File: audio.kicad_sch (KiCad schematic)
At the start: 69 parts, among them U10 OPA1642, U17 DG413xUE, U4 OPA1692xD, U5 OPA1692xD, U7 OPA1692xD, U8 OPA1692xD, U9 OPA1692xD

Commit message: modified:   MCU.kicad_sch 	modified:   PSU.kicad_sch 	modified:   ProjectY.kicad_pro 	modified:   ProjectY.kicad_sch 	modified:   ad.kicad_sch 	modified:   audio.kicad_sch
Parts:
- removed R25, R26: 4.7k, symbol Device:R
- removed U10: OPA1642, Package_SO:SOIC-8_3.9x4.9mm_P1.27mm, symbol Amplifier_Operational:OPA1692xD
- removed U17: DG413xUE, Package_SO:TSSOP-16_4.4x5mm_P0.65mm, symbol Analog_Switch:DG413xUE
- removed U9: OPA1692xD, Package_SO:SOIC-8_3.9x4.9mm_P1.27mm, symbol Amplifier_Operational:OPA1692xD
- added C1: 10u, symbol Device:C_Polarized
- added C13, C23: 1uF, PCM_JLCPCB:C_0402, symbol PCM_JLCPCB-Capacitors:0402,1uF
- added C21, C22: 10uF, PCM_JLCPCB:C_0402, symbol PCM_JLCPCB-Capacitors:0402,10uF
- added U6: TAC5242, Package_DFN_QFN:VQFN-24-1EP_4x4mm_P0.5mm_EP2.5x2.5mm_ThermalVias, symbol User:TAC5242
- added U9: OPA2156xD, Package_SO:SOIC-8_3.9x4.9mm_P1.27mm, symbol Amplifier_Operational:OPA2156xD
- R19, R20: value 4.7k -> 10k
- R23, R24: value 4.7k -> 2Meg
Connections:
- net VREF is gone; now on net +3.5VA: U8.3 (+), U8.5 (+)
- net ADC_L+: now also U6.15 (IN1P)
- net ADC_L-: now also U6.16 (IN1M)
- net ADC_R+: now also U6.17 (IN2P)
- net ADC_R-: now also U6.18 (IN2M)
- net DAC_L+: now also U6.20 (OUT1P)
- net DAC_L-: now also U6.19 (OUT1M)
- net DAC_R+: now also U6.21 (OUT2P)
- net DAC_R-: now also U6.22 (OUT2M)
- net GND: now also R20.2, R23.2, R24.2, C1.2, C13.2, C21.2, C22.2, C23.2, U6.10 (MD4), U6.12 (MD5), U6.13 (MD0), U6.25 (EPAD), U6.9 (MD3), U6.A1 (VSS), U6.A2 (VSS), U6.A3 (VSS), U6.A4 (VSS), U9.4 (V-); no longer R22.2, R28.2, R30.2, R32.2, R34.2, R8.2
- net Guitar_IN_L: now also R23.1
- net Guitar_IN_R: now also R24.1
- net at C34.2, R3.2, U7.1: now also R41.1; no longer R20.1
- net at C31.2, R14.2, R8.1: now also U9.3 (+)
- net at R15.1, R27.1: now also U9.1, U9.2 (-)
- net at C33.2, R21.2, R22.1: now also U9.5 (+)
- net at R17.1, R31.1: now also U9.6 (-), U9.7
- net at C39.2, R13.2, U7.7: now also R42.1; no longer R24.1
- net +3.5VA: now reaches R19.2
- net +3.5VA: now also R20.1, R22.2, R28.2, R30.2, R32.2, R34.2, R8.2, C1.1; no longer R41.1
- net +7VA: now reaches R19.1
- net +7VA: now also U9.8 (V+); no longer R20.2
- net ADC_DRV_OUT_L-: no longer names the net of R16.1, R29.1, U8.1
- net ADC_DRV_OUT_L-: no longer R23.2
- net ADC_DRV_OUT_R-: no longer names the net of R18.1, R33.1, U8.7
- new net: C13.1, U6.14 (MICBIAS)
- new net: C22.1, U6.1 (DREG)
- new net: C23.1, U6.24 (VREF)
- new net 3.3V: C21.1, U6.6 (IOVDD)
- new net 3.3VA: U6.23 (AVDD), U6.7 (MD1), U6.8 (MD2)
- new net GP0: U6.11 (GPO)
- new net I2S_CK: U6.2 (BCLK)
- new net I2S_SDI: U6.4 (DOUT)
- new net I2S_SDO: U6.5 (DIN)
- new net I2S_WS: U6.3 (FSYNC)
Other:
- moved on the sheet: C27, C28, C29, C30, C34, C35, C36, C37, C38, C39, R1, R10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

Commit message: modified:   MCU.kicad_sch 	modified:   PSU.kicad_sch 	modified:   ProjectY.kicad_pro 	modified:   ProjectY.kicad_sch 	modified:   audio.kicad_sch 	modified:   fp-info-cache 	new file:   spdif.kicad_sch 	modified:   usbfilter.kicad_sch
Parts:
- removed C1: 10u, symbol Device:C_Polarized
- removed C34, C38, C39: 330p, symbol Device:C
- removed C35, C36: 100u, symbol Device:C
- removed C37, C44, C45: 2.2n, symbol Device:C
- removed R10, R13: 4.7k, symbol Device:R
- removed R11, R12: 200, symbol Device:R
- removed R19, R20: 10k, symbol Device:R
- removed R45, R46: 100, symbol Device:R
- removed U4, U5, U7, U8: OPA1692xD, Package_SO:SOIC-8_3.9x4.9mm_P1.27mm, symbol Amplifier_Operational:OPA1692xD
- added C1, C11, C12, C15, C16, C17, C18, C19, C2, C20: 100nF, PCM_JLCPCB:C_0402, symbol PCM_JLCPCB-Capacitors:0402,100nF
- added C36, C37, C38, C39, C44, C45: 2.2nF, PCM_JLCPCB:C_0805, symbol PCM_JLCPCB-Capacitors:0805,2.2nF
- added D2, D3, D4, D5, D6, D7: BAV99,215, PCM_JLCPCB:SOT-23-3_L2.9-W1.6-P1.90-LS2.8-BR, symbol PCM_JLCPCB-Diode-Packages:Switching, BAV99,215
- added R43, R44: 600 0.1%, symbol Device:R
- added U10, U14: OPA1692xDGK, Package_SO:VSSOP-8_3x3mm_P0.65mm, symbol Amplifier_Operational:OPA1692xDGK
- added U7, U8: OPA2156xD, Package_SO:SOIC-8_3.9x4.9mm_P1.27mm, symbol Amplifier_Operational:OPA2156xD
- C29: value 2.2n -> 100u
- C30: value 330p -> 100u
- R1, R2: value 4.7k -> 1k 0.1%
- R15, R16, R17, R18: value 4.7k -> 2.2k
- R27, R28, R29, R30, R31, R32, R33, R34: value 2.2k -> 1k
- R3, R6, R7, R9: value 4.7k -> ?
- R4, R5: value 200 -> 1k 0.1%
- R41, R42: value 100 -> 600 0.1%
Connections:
- net +3.5VA: now also U8.3 (+), U8.5 (+); no longer R22.2, R28.2, R30.2, R32.2, R34.2, R8.2
- net DAC_R+: now also C30.2
- net DAC_R-: now also C29.1
- net GND: now also R22.2, R28.2, R30.2, R32.2, R34.2, R42.1, R7.1, R8.2, C1.2, C11.2, C12.1, C15.2, C16.1, C17.2, C18.1, C19.2, C2.1, C20.1, R44.1; no longer C30.2, U9.4 (V-)
- net Guitar_IN_L: now also D2.3
- net Guitar_IN_R: now also D3.3
- net Line_Output_L+: now also D4.3
- net Line_Output_L-: now also R42.2, D5.3
- net Line_Output_R+: now also D6.3, R43.2; no longer R42.2
- net Line_Output_R-: now also D7.3, R44.2
- net at R1.2, R3.1: now also C38.2, C39.2, U7.2 (-); no longer C29.1, R4.1
- net at R3.2, R41.1: now also U7.1
- net at R27.2, R28.1: now also U10.5 (+)
- net at R7.2: now also R5.2, C44.1, C45.1, U7.5 (+)
- net at R31.2, R32.1: now also U14.5 (+)
- net at R2.2, R6.2: now also C38.1, C39.1, U7.3 (+); no longer C29.2, R5.1
- net at C46.1, R37.2: now also C37.2
- net at C47.2, R38.2: now also C37.1
- net at R4.2: now also R9.1, C44.2, C45.2, U7.6 (-)
- net at R18.1, R33.1: now also U8.7
- net at R33.2, R34.1: now also U14.3 (+)
- net at R9.2: now also R43.1, U7.7
- net at R16.1, R29.1: now also U8.1
- net at R15.2, R16.2: now also U8.2 (-)
- net at R37.1: now also U14.1, U14.2 (-)
- net at R29.2, R30.1: now also U10.3 (+)
- net at R38.1: now also U14.6 (-), U14.7
- net at R17.2, R18.2: now also U8.6 (-)
- net at C30.1: now also R5.1; no longer R5.2
- net at C40.1, R35.2: now also C36.2
- net at C43.2, R36.2: now also C36.1
- net at R36.1: now also U10.6 (-), U10.7
- net at R35.1: now also U10.1, U10.2 (-)
- net +7VA renamed +5V
- net +5V: now also C1.1, C11.1, C15.1, C17.1, C19.1, D2.2, D3.2, D4.2, D5.2, D6.2, D7.2, U10.8 (V+), U14.8 (V+), U7.8 (V+), U8.8 (V+)
- new net: C29.2, R4.1
- new net -5V: C12.2, C16.2, C18.2, C2.2, C20.2, D2.1, D3.1, D4.1, D5.1, D6.1, D7.1, U10.4 (V-), U14.4 (V-), U7.4 (V-), U8.4 (V-), U9.4 (V-)
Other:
- moved on the sheet: C13, C21, C22, C23, C27, C28, C31, C32, C33, C40, C43, C46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

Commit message: asd
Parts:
- removed C31, C33: 100p, symbol Device:C
- removed C32, C8: 1u, symbol Device:C
- removed D2, D3, D4, D5, D6, D7: BAV99,215, PCM_JLCPCB:SOT-23-3_L2.9-W1.6-P1.90-LS2.8-BR, symbol PCM_JLCPCB-Diode-Packages:Switching, BAV99,215
- removed R1, R2, R4, R5: 1k 0.1%, symbol Device:R
- removed R14, R21, R35, R36, R37, R38: 100, symbol Device:R
- removed R15, R16, R17, R18: 2.2k, symbol Device:R
- removed R22, R23, R24, R8: 2Meg, symbol Device:R
- removed R27, R28, R29, R30, R31, R32, R33, R34: 1k, symbol Device:R
- removed U7: OPA2156xD, Package_SO:SOIC-8_3.9x4.9mm_P1.27mm, symbol Amplifier_Operational:OPA2156xD
- added C31, C32, C70, C71, C72, C8, C81, C82, C83, C84: 100nF, PCM_JLCPCB:C_0402, symbol PCM_JLCPCB-Capacitors:0402,100nF
- added C34, C35, C85, C86, C87, C94: 100pF, PCM_JLCPCB:C_0402, symbol PCM_JLCPCB-Capacitors:0402,100pF
- added D11, D12, D13, D14, D15, D16, D17, D18, D19, D8: BAV99, Package_TO_SOT_SMD:SOT-23, symbol Diode:BAV99
- added K1, K2, K3, K4: G6K-2, symbol Relay:G6K-2
- added Q6, Q7, Q8, Q9: BC847, Package_TO_SOT_SMD:SOT-23, symbol Transistor_BJT:BC847
- added R100, R103, R68, R71: 10kΩ, PCM_JLCPCB:R_0402, symbol PCM_JLCPCB-Resistors:0402,10kΩ
- added R101, R102, R20, R21, R22, R23, R26, R27, R28, R29, R31, R32, R33, R34, R37, R38, R62, R63, R64, R65, R66, R67, R72, R73, R76, R77: 1kΩ, PCM_JLCPCB:R_0805, symbol PCM_JLCPCB-Resistors:0805,1kΩ
- added R13, R14, R16, R24, R25, R69, R70, R80, R81, R98: 100Ω, PCM_JLCPCB:R_0805, symbol PCM_JLCPCB-Resistors:0805,100Ω
- added R17, R18: 2.2kΩ, PCM_JLCPCB:R_0805, symbol PCM_JLCPCB-Resistors:0805,2.2kΩ
- added R75, R79, R82, R83: 510Ω, PCM_JLCPCB:R_0805, symbol PCM_JLCPCB-Resistors:0805,510Ω
- added R8, R99: 1MΩ, PCM_JLCPCB:R_0805, symbol PCM_JLCPCB-Resistors:0805,1MΩ
- added R88, R89, R90, R91: 10kΩ, PCM_JLCPCB:R_0805, symbol PCM_JLCPCB-Resistors:0805,10kΩ
- added U13, U16, U23, U5: OPA2156xD, Package_SO:SOIC-8_3.9x4.9mm_P1.27mm, symbol Amplifier_Operational:OPA2156xD
- added U24: OPA1692xDGK, Package_SO:VSSOP-8_3x3mm_P0.65mm, symbol Amplifier_Operational:OPA1692xDGK
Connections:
- net +3.5VA is gone; now on net GND: U8.3 (+), U8.5 (+)
- net DAC_R+: now also C29.1; no longer C30.2
- net DAC_R-: now also C30.2; no longer C29.1
- net GND: now also C31.2, C32.1, C34.2, C35.2, C70.2, C71.1, C72.2, C8.2, C81.1, C82.2, C83.1, C84.1, C85.2, C86.2, C87.2, C94.2, Q6.2 (E), Q7.2 (E), Q8.2 (E), Q9.2 (E), R20.2, R23.2, R32.2, R34.2, R79.1, R8.2, R83.2, R88.2, R89.1, R90.2, R91.1, R99.2, U5.3 (+), U5.5 (+)
- net Line_Output_L+: now also D12.3 (K)
- net Line_Output_L-: now also D13.3 (K)
- net Line_Output_R+: now also D14.3 (K)
- net Line_Output_R-: now also D15.3 (K)
- net at C38.2, C39.2, R3.1: now also R26.2, U24.2 (-)
- net at R3.2: now also R62.2, U24.1; no longer R41.1
- net at C38.1, C39.1, R6.2: now also R27.2, U24.3 (+)
- net at U9.3 (+): now also C34.1, R13.2, R8.1
- net Unbal_Left: now reaches U9.1, U9.2 (-)
- net Unbal_Left: now also K2.5
- net at U10.5 (+): now also R20.1, R21.2
- net at U9.5 (+): now also C94.1, R98.2, R99.1
- net at C44.2, C45.2, R9.1: now also R28.2, U24.6 (-)
- net at R9.2: now also R64.2, U24.7; no longer R43.1
- net Unbal_Right: now reaches U9.6 (-), U9.7
- net Unbal_Right: now also K2.4
- net at U14.5 (+): now also R33.2, R34.1
- net at C30.1: now also R29.1
- net at C27.2: now also R26.1
- net Processing_Inverted_Right: now reaches U8.7
- net Processing_Inverted_Right: now also R18.2, R31.1, R66.1
- net at U14.3 (+): now also R31.2, R32.1
- net at C44.1, C45.1, R7.2: now also R29.2, U24.5 (+)
- net Processing_Inverted_Left: now reaches U8.1
- net Processing_Inverted_Left: now also R101.1, R102.1, R22.1, R67.1, R77.2
- net at U8.2 (-): now also R76.1, R77.1
- net at U14.6 (-), U14.7: now also R70.1
- net at U10.3 (+): now also R22.2, R23.1
- net at U14.1, U14.2 (-): now also R69.1
- net at C37.2, C46.1: now also R69.2
- net at U10.6 (-), U10.7: now also R25.1
- net at C28.1: now also R27.1
- net at U8.6 (-): now also R17.2, R18.1
- net at C36.1, C43.2: now also R25.2
- net at C36.2, C40.1: now also R24.2
- net at C29.2: now also R28.1
- net at U10.1, U10.2 (-): now also R24.1
- net at C37.1, C47.2: now also R70.2
- net +5V renamed +4.5V
- net +4.5V: now also C31.1, C70.1, C72.1, C8.1, C82.1, D11.2 (A), D12.2 (A), D13.2 (A), D14.2 (A), D15.2 (A), D16.2 (A), D17.2 (A), D18.2 (A), D19.2 (A), D8.2 (A), U13.8 (V+), U16.8 (V+), U23.8 (V+), U24.8 (V+), U5.8 (V+)
- net -5V renamed -4.5V
- net -4.5V: now also C32.2, C71.2, C81.2, C83.2, C84.2, D11.1 (K), D12.1 (K), D13.1 (K), D14.1 (K), D15.1 (K), D16.1 (K), D17.1 (K), D18.1 (K), D19.1 (K), D8.1 (K), U13.4 (V-), U16.4 (V-), U23.4 (V-), U24.4 (V-), U5.4 (V-)
- net 3.3V renamed +3.3V
- net +3.3V: now also K1.1, K2.1, K3.1, K4.1
- net 3.3VA renamed +3.3VA
- new net: Q7.1 (B), R71.2
- new net: K2.8, Q7.3 (C)
- new net: C86.1, R80.2, R90.1, U23.3 (+)
- new net: R37.2, R75.1, U16.2 (-)
- new net: R38.2, R79.2, U16.3 (+)
- new net: C35.1, R14.2, R88.1, U13.3 (+)
- new net: C85.1, R16.2, R89.2, U13.5 (+)
- new net: R37.1, U13.1, U13.2 (-)
- new net: Q9.1 (B), R103.2
- new net: K4.8, Q9.3 (C)
- new net: C87.1, R81.2, R91.2, U23.5 (+)
- new net: R73.1, U23.6 (-), U23.7
- new net: K1.6, R66.2
- new net: Q8.1 (B), R68.2
- new net: K1.8, Q8.3 (C)
- new net: R43.1, R65.1, U5.1
- new net: R64.1, R65.2, U5.2 (-)
- new net: R72.1, U23.1, U23.2 (-)
- new net: Q6.1 (B), R100.2
- new net: R38.1, U13.6 (-), U13.7
- new net: R41.1, R63.1, U5.7
- new net: K4.3, R101.2
- new net: K4.6, R102.2
- new net: K1.3, R67.2
- new net: R73.2, R83.1, U16.5 (+)
- new net: K3.8, Q6.3 (C)
- new net: R72.2, R82.2, U16.6 (-)
- new net Balun_In_Left+: D16.3 (K), K3.5, R16.1
- new net Balun_In_Left-: D8.3 (K), K3.4, R14.1
- new net Balun_Left: K2.7, R75.2, U16.1
- new net Balun_Right: K2.2, R82.1, U16.7
- new net Buffer_In_Left: D11.3 (K), K3.7, R13.1
- new net Buffer_In_Right: D19.3 (K), K3.2, R98.1
- new net Dry_Through: R68.1
- new net Hi-Z: R71.1
- new net IN_L+: K3.6
- new net IN_L-: K3.3
- new net IN_R+: D18.3 (K), R81.1
- new net IN_R-: D17.3 (K), R80.1
- new net Mono_Dry_Through: R103.1
- new net Processing_In_Left: K2.6, R21.1, R76.2
- new net Processing_In_Right: K2.3, R17.1, R33.1
- new net Summing_In_L: K1.4, K4.4, R62.1, R63.2, U5.6 (-)
- new net Summing_In_R: K1.5, K4.5
- new net ~{Hi-Z2}: R100.1
- no-connect marks 0 -> 4
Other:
- moved on the sheet: C1, C11, C12, C13, C15, C16, C17, C18, C19, C2, C20, C21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

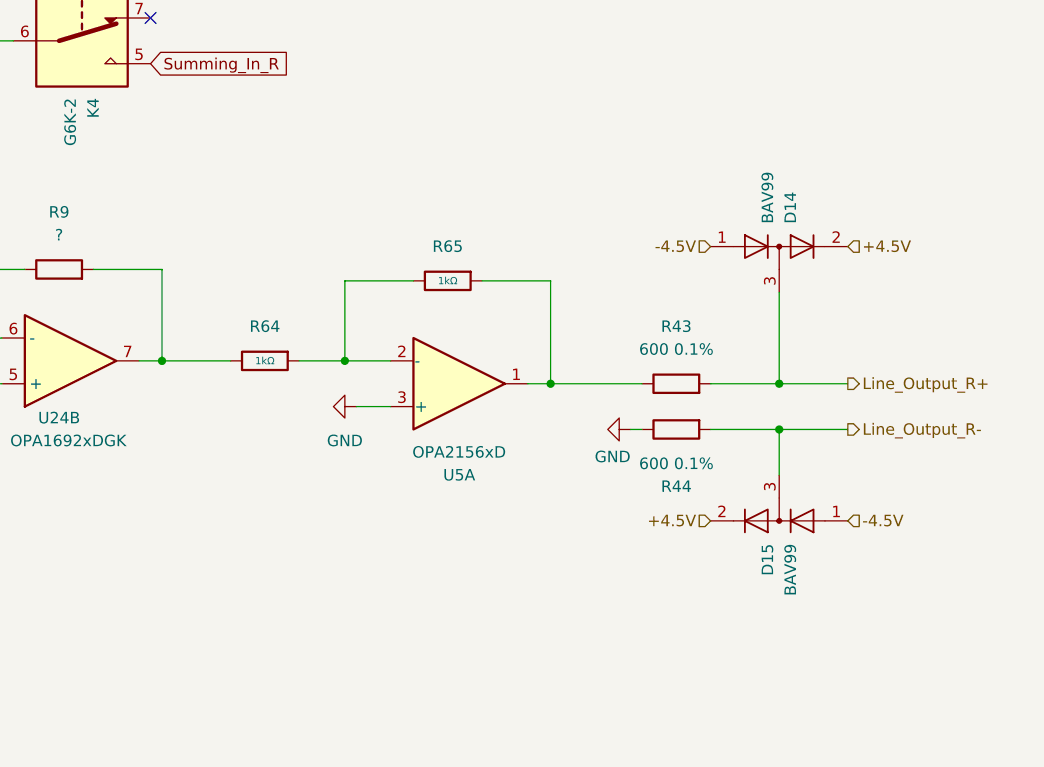
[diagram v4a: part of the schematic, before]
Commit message: commit
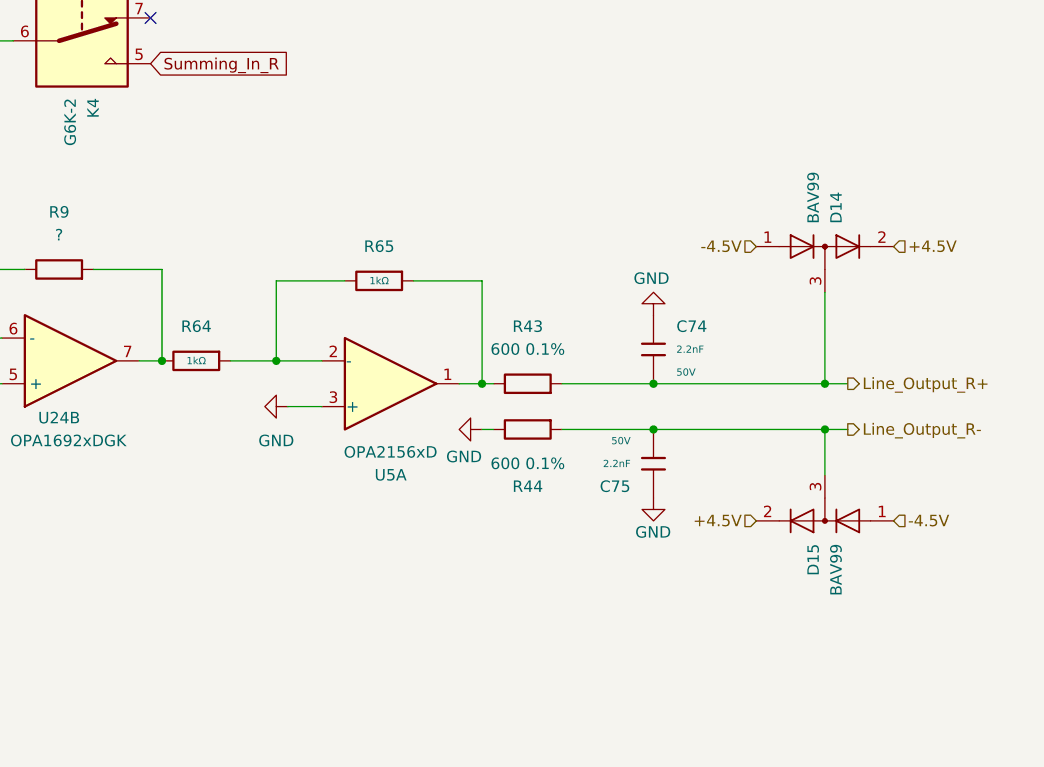
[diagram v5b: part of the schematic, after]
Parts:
- added C74, C75: 2.2nF, PCM_JLCPCB:C_0805, symbol PCM_JLCPCB-Capacitors:0805,2.2nF
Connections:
- net GND: now also C74.1, C75.1
- net Line_Output_R+: now also C74.2
- net Line_Output_R-: now also C75.2
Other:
- moved on the sheet: D14, D15, R43, R44, R64, R65, U5A
